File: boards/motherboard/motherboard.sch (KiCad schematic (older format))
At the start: 40 parts, among them J1 RJ45, J2 RJ45, J3 RJ45, J4 RJ45, J5 RJ45, U1 EBAYPCA9685

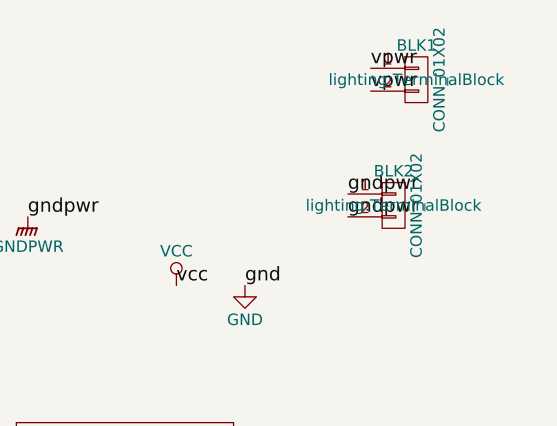
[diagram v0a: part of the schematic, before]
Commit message: another revision
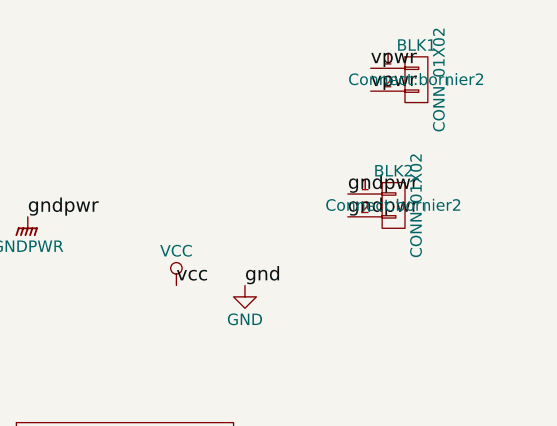
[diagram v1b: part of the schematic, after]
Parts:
- BLK1, BLK2: footprint lighting:TerminalBlock -> Connect:bornier2
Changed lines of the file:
@@
 F 0 "BLK1" H 10850 800 50  0000 C CNN
 F 1 "CONN_01X02" V 10950 650 50  0000 C CNN
-F 2 "lighting:TerminalBlock" H 10850 650 50  0000 C CNN
+F 2 "Connect:bornier2" H 10850 650 50  0000 C CNN
 F 3 "" H 10850 650 50  0000 C CNN
 	1    10850 650
@@
 F 0 "BLK2" H 10750 1350 50  0000 C CNN
 F 1 "CONN_01X02" V 10850 1200 50  0000 C CNN
-F 2 "lighting:TerminalBlock" H 10750 1200 50  0000 C CNN
+F 2 "Connect:bornier2" H 10750 1200 50  0000 C CNN
 F 3 "" H 10750 1200 50  0000 C CNN
 	1    10750 1200

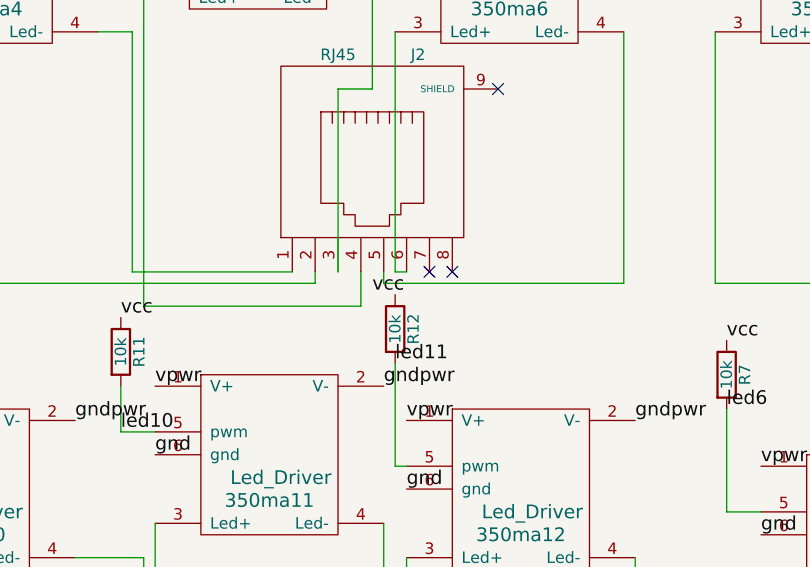
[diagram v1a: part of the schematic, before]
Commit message: minor fix
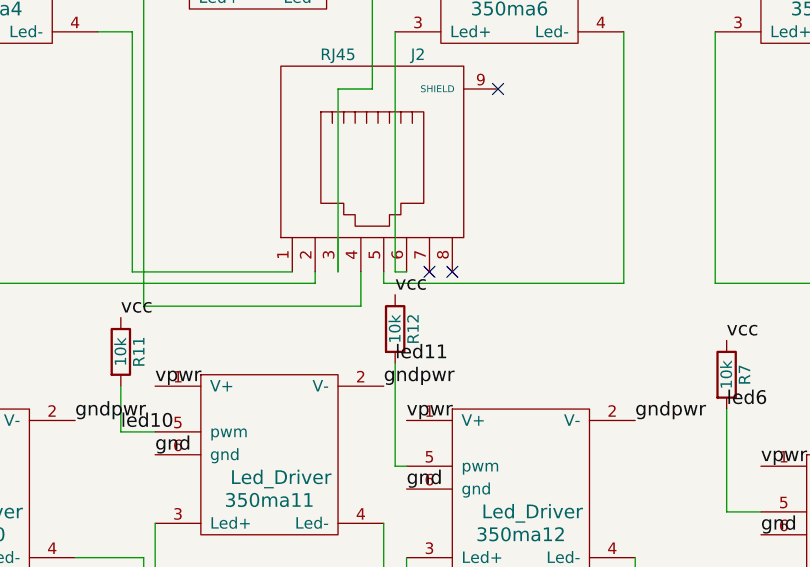
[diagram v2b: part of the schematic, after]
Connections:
- net VCC: now also R12.1
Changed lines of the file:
@@
 	1    0    0    -1
 $EndComp
-Text Label 3050 2950 0    60   ~ 0
+Text Label 3150 2950 0    60   ~ 0
 vcc
 $Comp
